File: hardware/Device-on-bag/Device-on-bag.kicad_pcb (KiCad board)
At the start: 2 copper layers, 67.3 x 56.5 mm, 5 parts, among them J1 Conn_01x08, J2 Conn_01x08, J3 Conn_01x12, J4 Conn_01x12, U2 ESP32-DEVKIT-V1

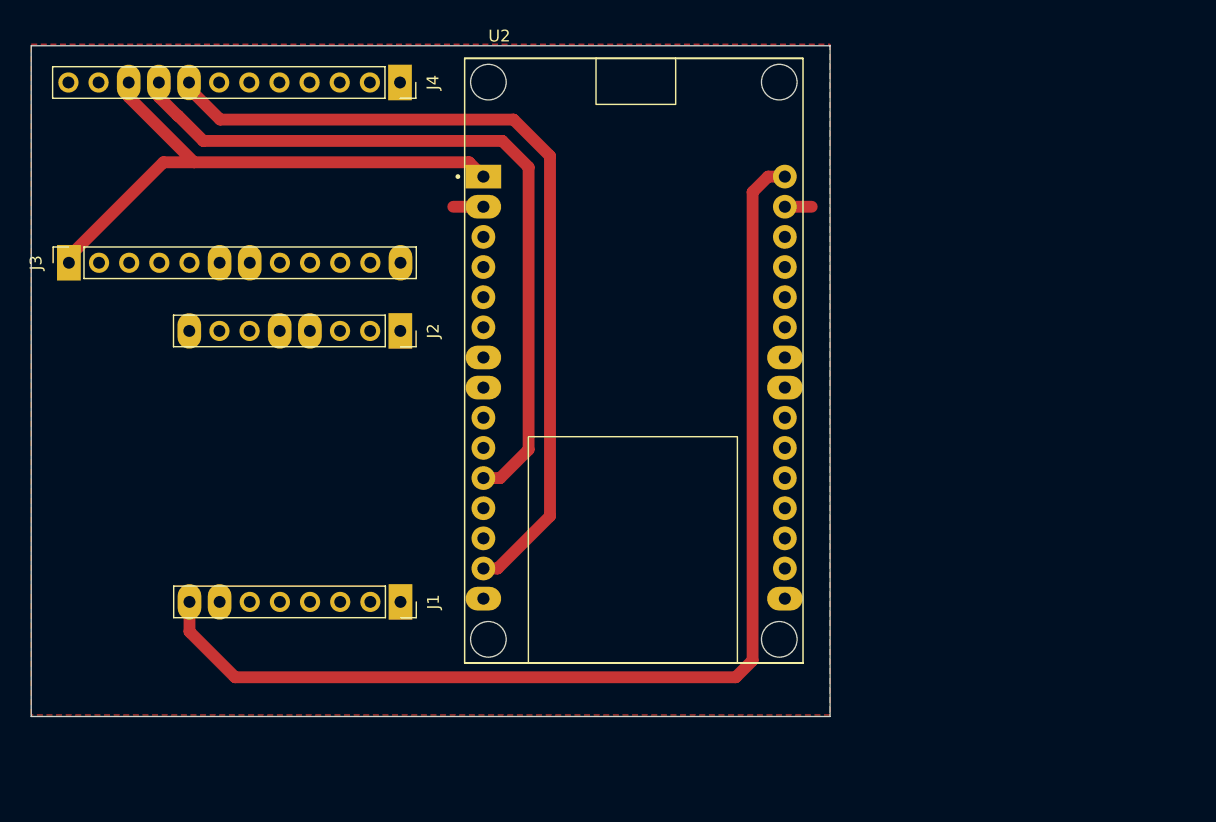
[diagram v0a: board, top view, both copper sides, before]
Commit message: update
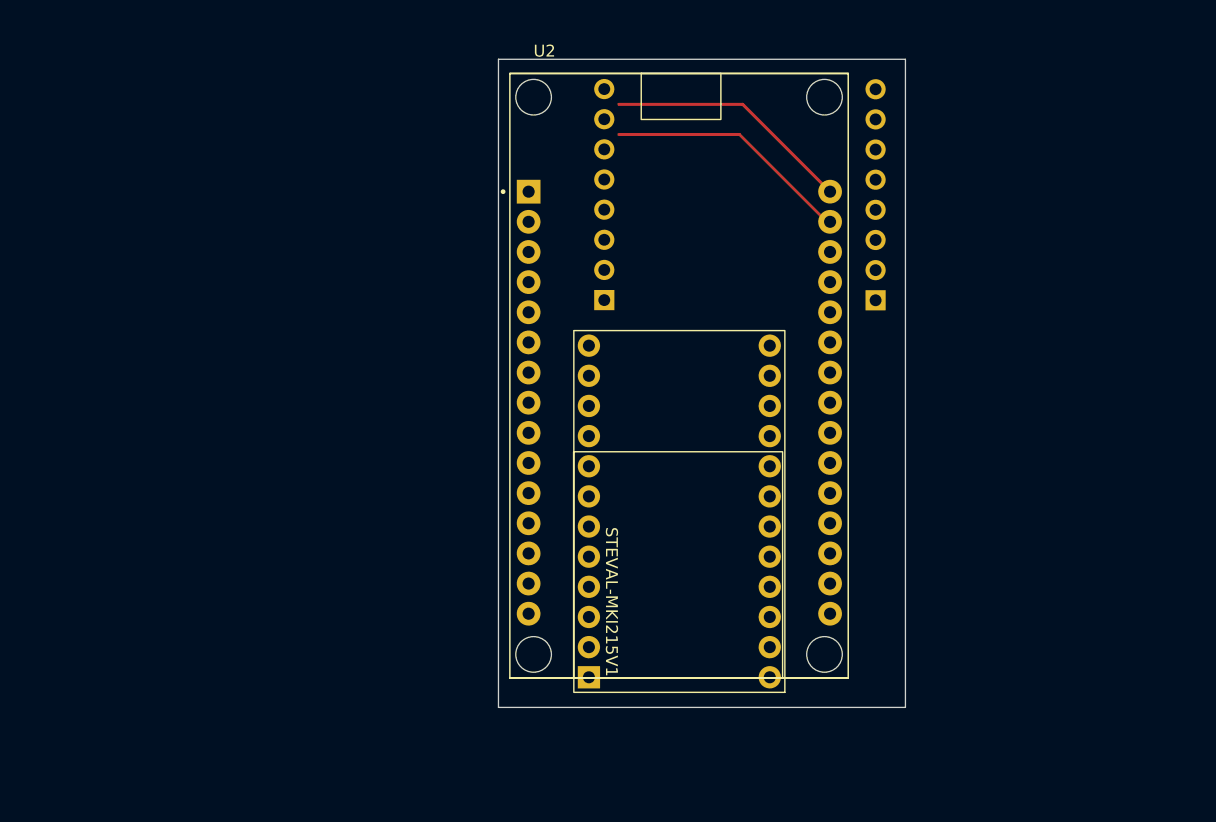
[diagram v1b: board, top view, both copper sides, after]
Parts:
- removed J3, J4: Conn_01x12, Connector_PinSocket_2.54mm:PinSocket_1x12_P2.54mm_Vertical
- added U1: STEVAL-MKI215V1, STEVAL-MKI215V1:STEVAL-MKI215V1, B.Cu at (97.8, 66.0)
- J1, J2: moved to B.Cu
- moved J2 40.1 mm to (114.3, 48.2), turned to 0 degrees
- moved J1 30.7 mm to (91.5, 48.2), turned to 0 degrees
- moved U2 4.02 mm to (97.8, 54.6)
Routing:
- net Vin: track 94.8 -> 20.9 mm
- net SCL: track 71.8 -> 0.00 mm
- net SDA: track 63.4 -> 0.00 mm
- net 3.3V: track 48.2 -> 0.00 mm
- net GND: track 4.80 -> 20.9 mm
- removed copper zone on F.Cu, net GND
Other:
- board size 67.3 x 56.5 mm -> 34.3 x 54.6 mm

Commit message: update device on bag hardware
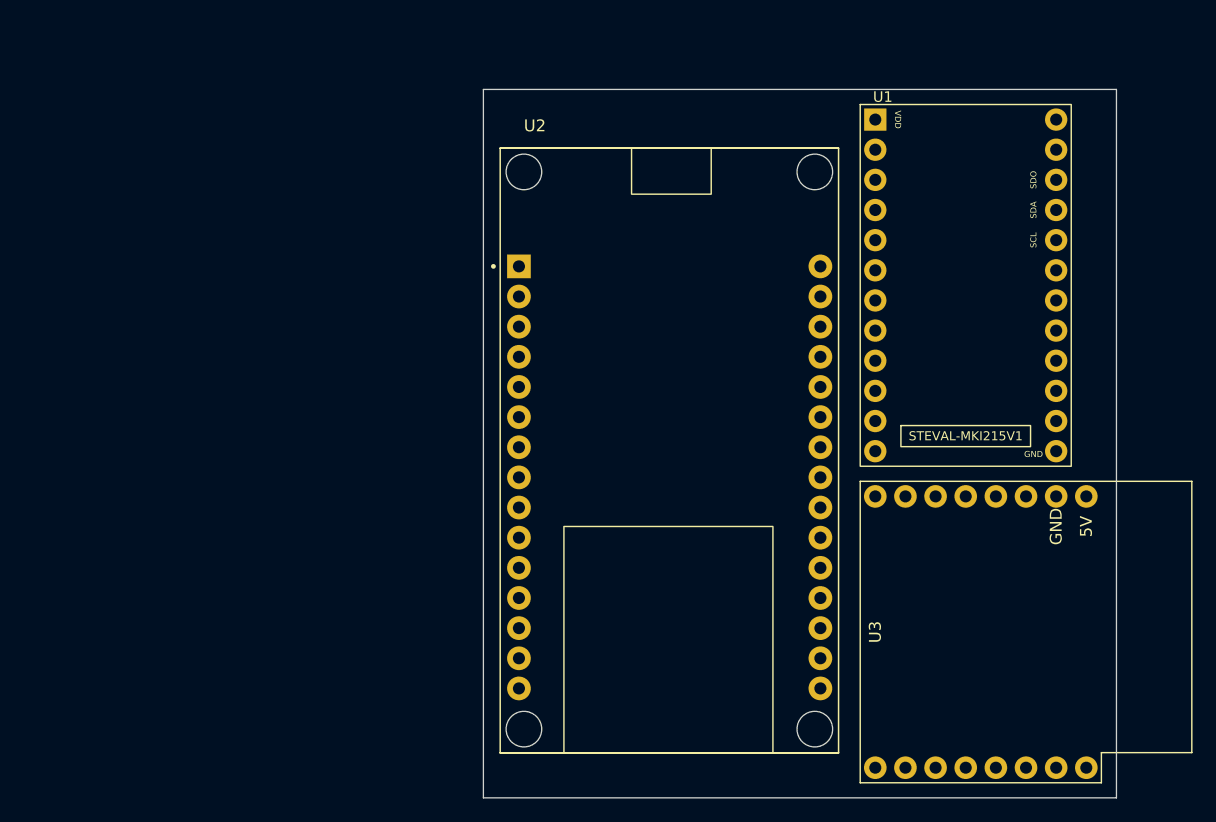
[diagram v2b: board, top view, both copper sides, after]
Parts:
- removed J1, J2: Conn_01x08, Connector_PinSocket_2.54mm:PinSocket_1x08_P2.54mm_Vertical
- added U3: D1_mini_battery_shield, D1 mini battery shield:D1 mini battery shield, F.Cu at (121.9, 76.2)
- U1: moved to F.Cu
- moved U1 30.7 mm to (121.9, 47.0)
- moved U2 6.35 mm to (97.0, 60.9)
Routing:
- net Vin: track 20.9 -> 0.00 mm
- net GND: track 20.9 -> 0.00 mm
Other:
- board size 34.3 x 54.6 mm -> 53.3 x 59.7 mm
